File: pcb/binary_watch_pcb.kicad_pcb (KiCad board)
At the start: 2 copper layers, 32.7 x 37.9 mm, 35 parts, among them IC1 ATMEGA168PA-A, SW1 SW_PUSH, SW2 SW_PUSH, X1 CRYSTAL

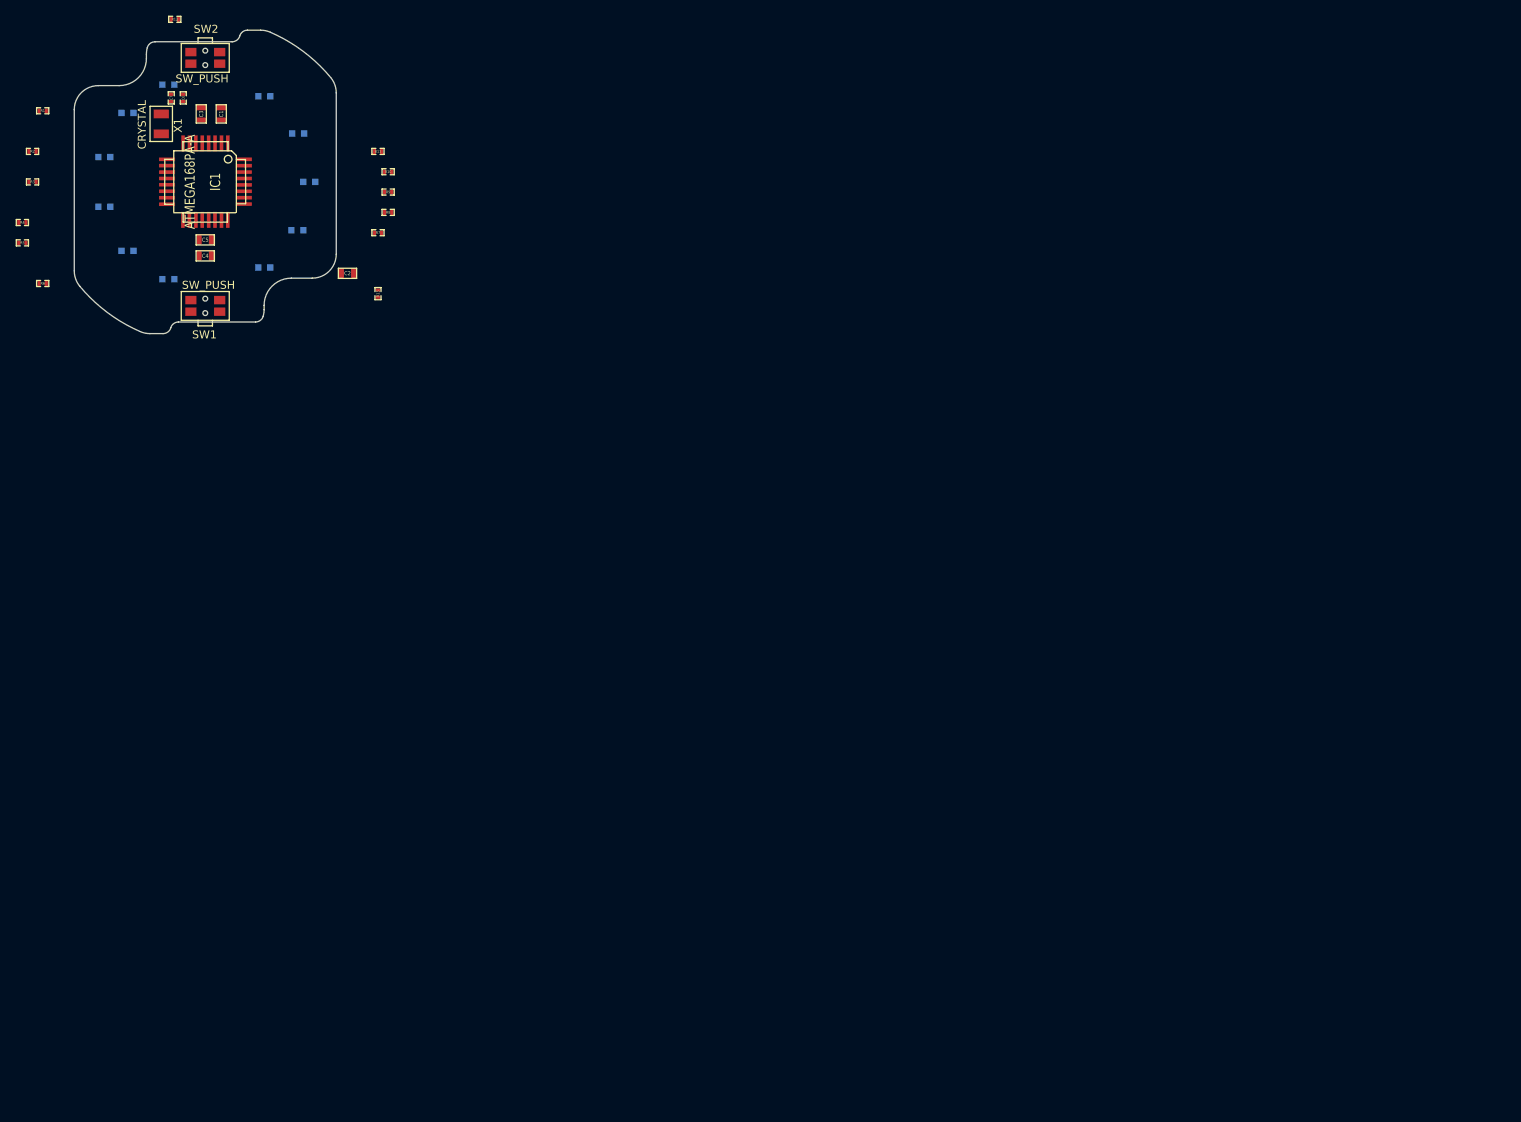
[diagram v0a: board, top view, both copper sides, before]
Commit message: Gen fab outputs, pdfs, and finish final routing.
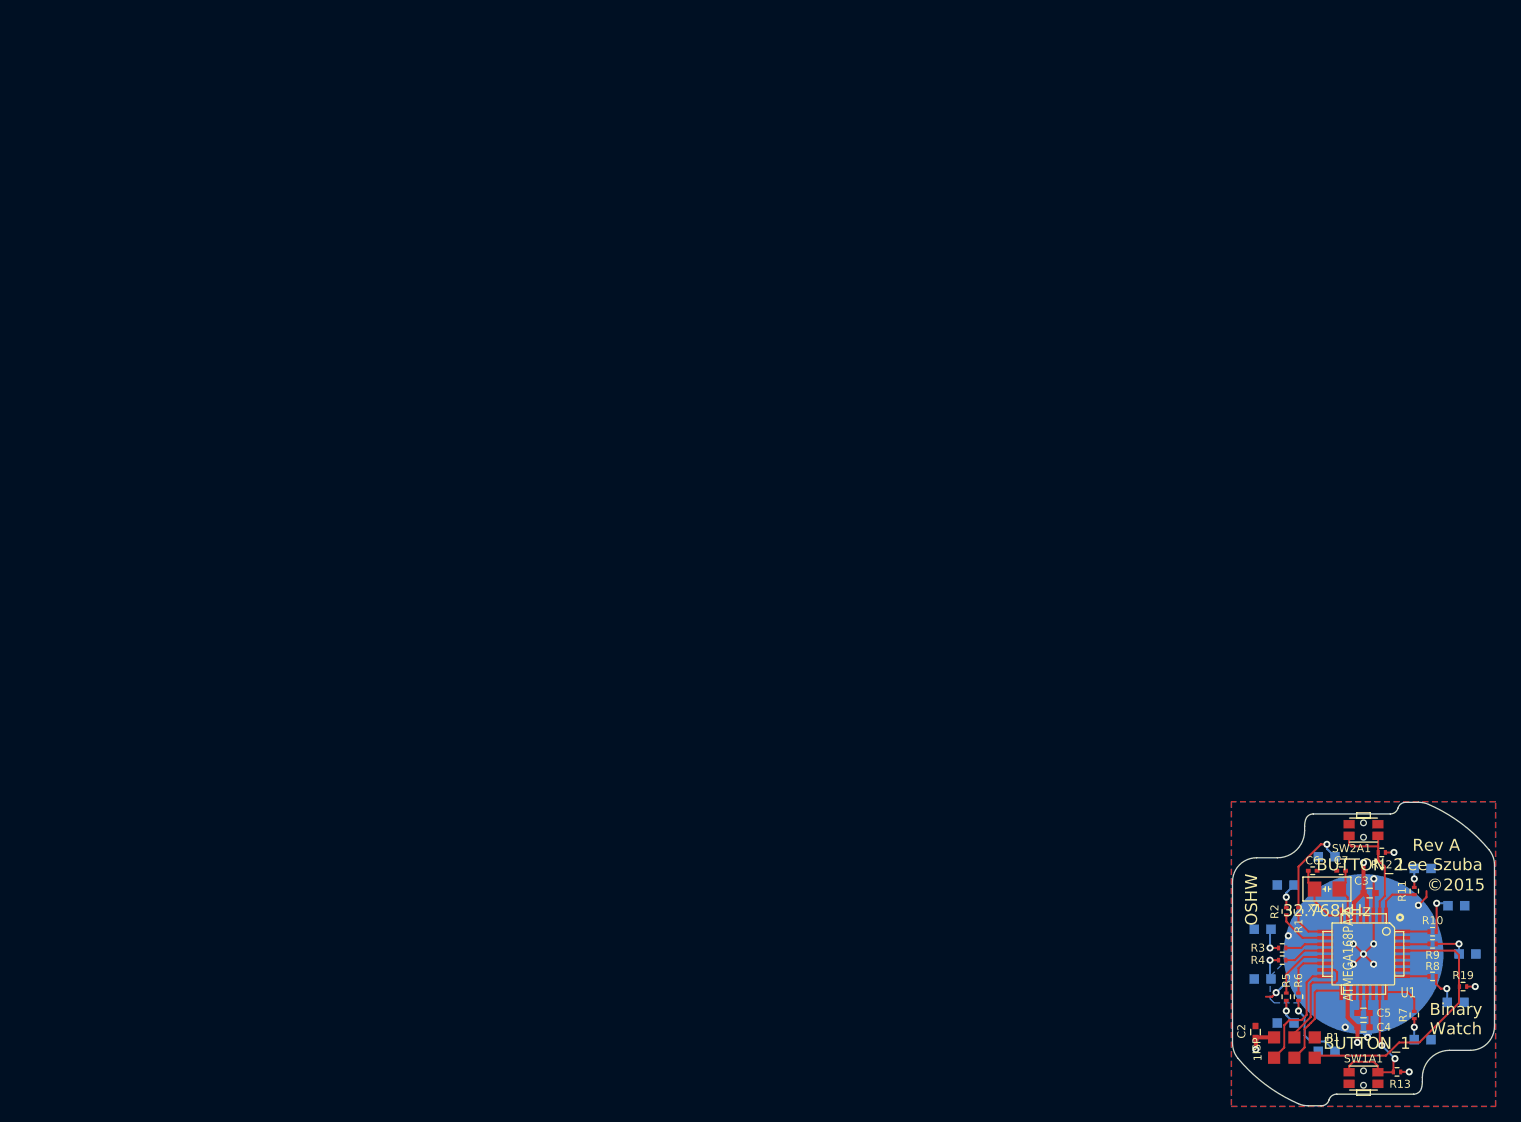
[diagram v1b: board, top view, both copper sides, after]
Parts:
- removed C1: 1uF, SM0603
- removed IC1: ATMEGA168PA-A, TQFP32
- removed SW1, SW2: SW_PUSH, EVQP7
- added BAT-N1: CONN_01X01, _ Custom Lib:CR2032-NEG, B.Cu at (144.8, 96.5)
- added P1: ISP, _ Custom Lib:HDR-2x3_SMD, F.Cu at (136.1, 108.2)
- added R19: 10k, Resistors_SMD:R_0402, F.Cu at (157.2, 100.6)
- added SW1A1: BUTTON_1, _ Custom Lib:EVQ-P7C01P, F.Cu at (144.8, 112.0)
- added SW2A1: BUTTON_2, _ Custom Lib:EVQ-P7C01P, F.Cu at (144.8, 81.0)
- added U1: ATMEGA168PA-A, _ Custom Lib:TQFP-32, F.Cu at (144.8, 96.5)
- C2, C3, C4, C5: footprint SM0603 -> Capacitors_SMD:C_0603
- C6, C7: value C -> 9pF; footprint SM0402 -> Capacitors_SMD:C_0402
- DH10, DH11, DH7, DH8, DH9, DM1, DM2, DM3, DM4, DM5, DM6: footprint LED-0603 -> LEDs:LED-0805
- R1, R10, R11, R12, R13, R2, R3, R4, R5, R6, R7, R8, R9: footprint SM0402 -> Resistors_SMD:R_0402
- X1: value CRYSTAL -> 32.768kHz; footprint ADS07 -> _ Custom Lib:XTAL_ABS07
- moved R1 186.2 mm to (136.7, 91.2), turned to 90 degrees
- moved R5 184.0 mm to (135.1, 101.9), turned to 270 degrees
- moved R12 183.3 mm to (147.1, 83.8)
- moved R2 183.3 mm to (135.1, 91.2), turned to 90 degrees
- moved R3 183.2 mm to (134.6, 95.8), turned to 180 degrees
- moved R4 182.5 mm to (134.6, 97.3), turned to 180 degrees
- moved R6 180.5 mm to (136.7, 101.9), turned to 270 degrees
- moved C3 175.5 mm to (145.5, 88.9), turned to 0 degrees
- moved C7 175.3 mm to (142.0, 86.1), turned to 180 degrees
- moved X1 174.3 mm to (140.2, 88.4), turned to 180 degrees
- moved C5 174.1 mm to (144.8, 103.9)
- moved DH11 174.0 mm to (152.2, 85.8)
- moved DH7 174.0 mm to (152.2, 107.2)
- moved DH8 174.0 mm to (156.3, 102.6)
- moved DH9 174.0 mm to (157.8, 96.5)
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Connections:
- net +3.3V renamed +BATT
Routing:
- net GND: track 0.00 -> 126.7 mm, vias 0 -> 11
- net /~RESET: track 0.00 -> 34.7 mm
- net +BATT: track 0.00 -> 23.9 mm, vias 0 -> 6
- net /SW_1: track 0.00 -> 18.7 mm, vias 0 -> 2
- net /SW_2: track 0.00 -> 17.5 mm
- net /MISO: track 0.00 -> 14.6 mm
- net /MOSI: track 0.00 -> 13.8 mm
- net /SCK: track 0.00 -> 12.7 mm
- net Net-(DM1-Pad2): track 0.00 -> 11.8 mm, vias 0 -> 1
- net Net-(DM6-Pad2): track 0.00 -> 9.33 mm, vias 0 -> 1
- net /XTAL2: track 0.00 -> 8.20 mm
- net /LED_M5: track 0.00 -> 8.13 mm
- net /LED_M6: track 0.00 -> 6.71 mm
- net /LED_M2: track 0.00 -> 6.54 mm
- net /XTAL1: track 0.00 -> 6.35 mm
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- added copper zone on B.Cu, net +BATT
- added copper zone on B.Cu, net GND
- added copper zone on F.Cu, net GND
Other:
- net class Default: via_drill 0.635 -> 0.508
- net class GND added: clearance 0.254, trace_width 0.508, via_dia 0.889, via_drill 0.508
- net class PWR added: clearance 0.254, trace_width 0.508, via_dia 0.889, via_drill 0.508
- board text added: "Binary Watch"
- board text added: "Lee Szuba"
- board text added: "OSHW"
- board text added: "Rev A"
- board text added: "©2015"
